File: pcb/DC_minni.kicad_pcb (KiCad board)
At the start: 4 copper layers, 72.2 x 87.7 mm, 60 parts, among them J1 DRUCKSENSOR, J2 Encoder, U1 ESP32-DevKitC, U2 USB-C to DIP PCB

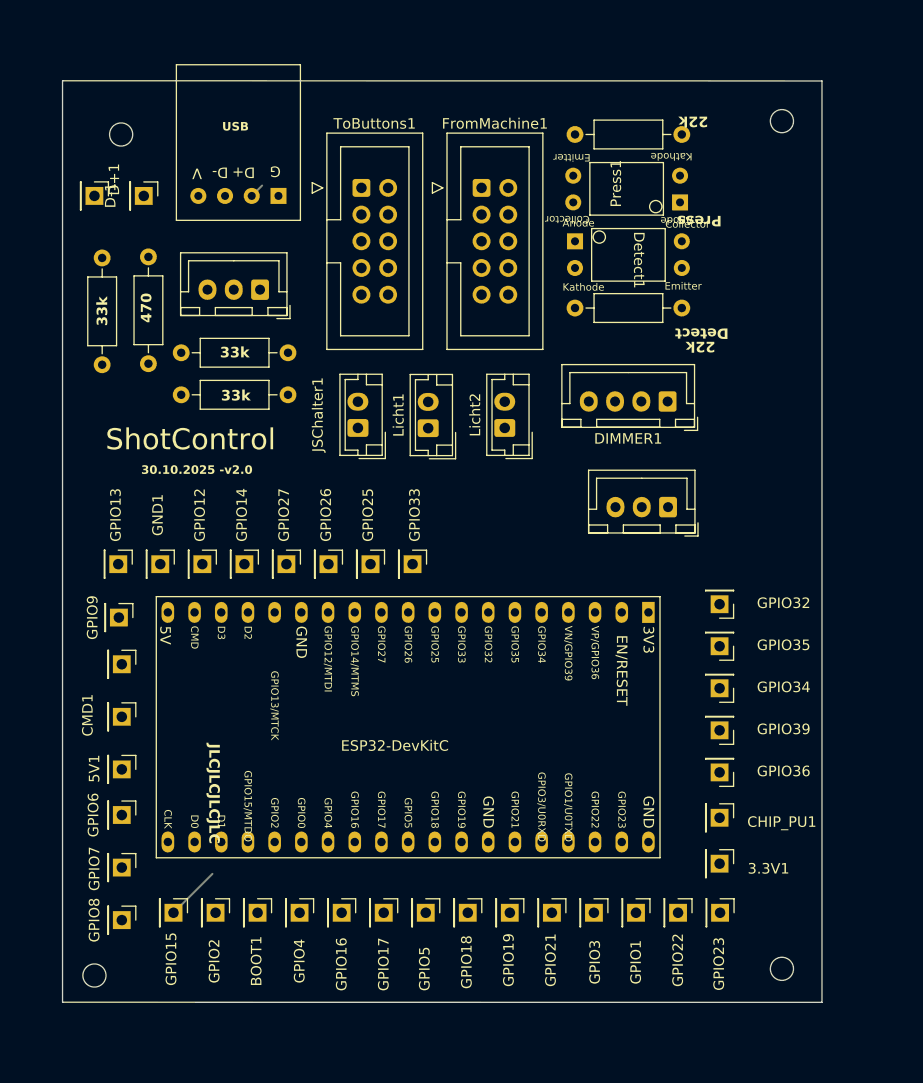
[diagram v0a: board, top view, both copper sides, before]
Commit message: PCB routing
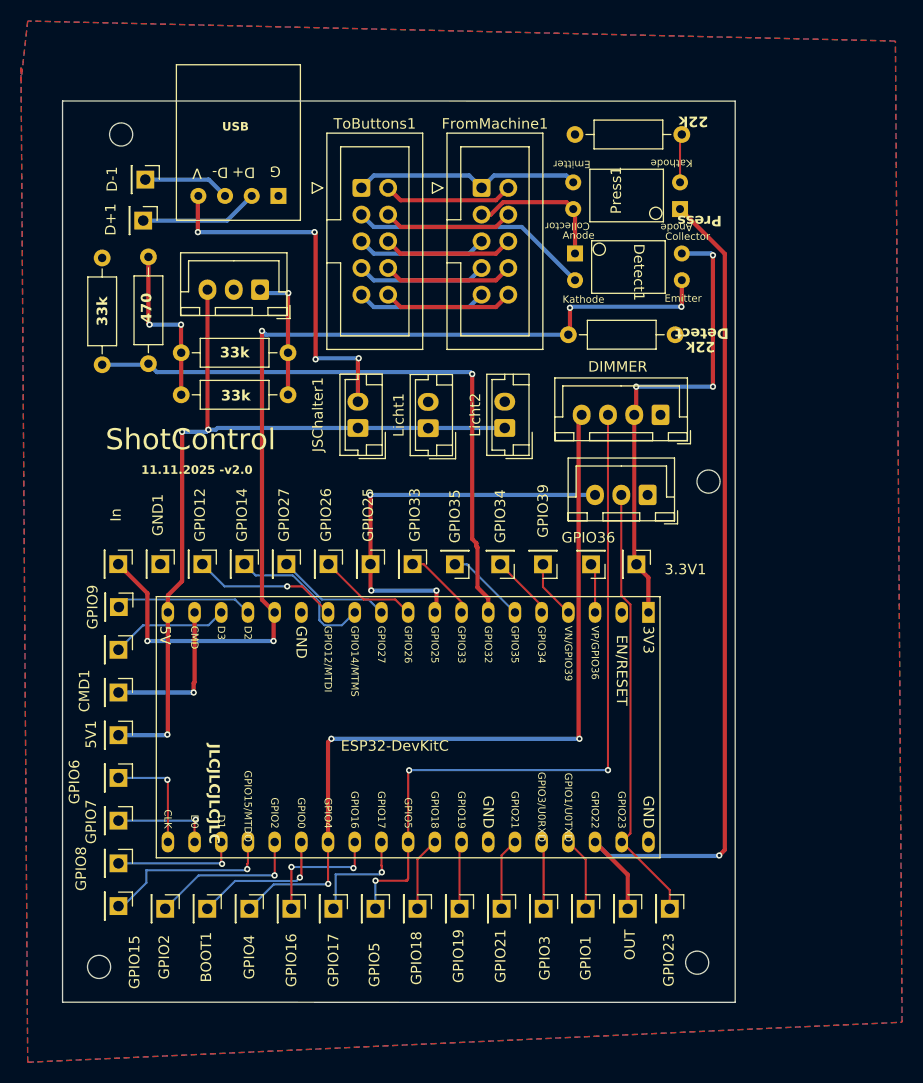
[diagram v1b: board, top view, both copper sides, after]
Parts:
- removed CHIP_PU1, GPIO32: Conn_01x01_Socket, Connector_PinHeader_2.54mm:PinHeader_1x01_P2.54mm_Vertical
- moved REF** 35.0 mm to (259.1, 113.0)
- moved 3.3V1 29.6 mm to (252.2, 120.9)
- moved GPIO35 26.4 mm to (234.9, 120.9)
- moved GPIO34 24.0 mm to (239.3, 120.9)
- moved GPIO36 23.3 mm to (247.9, 120.9)
- moved GPIO39 23.1 mm to (243.3, 120.9)
- moved REF** 8.09 mm to (258.0, 158.8)
- moved GPIO8 5.41 mm to (202.9, 149.4)
- moved GPIO15 5.27 mm to (202.9, 153.4)
- moved D+1 5.20 mm to (205.3, 88.2)
- moved BOOT1 4.80 mm to (211.4, 153.7)
- moved GPIO1 4.80 mm to (247.4, 153.7)
- moved GPIO16 4.80 mm to (219.4, 153.7)
- moved GPIO17 4.80 mm to (223.4, 153.7)
- moved GPIO18 4.80 mm to (231.4, 153.7)
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- renumbered DIMMER1 to DIMMER, GPIO13 to In, GPIO22 to OUT
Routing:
- net IN: track 0.00 -> 95.6 mm, vias 0 -> 5
- net OUT: track 0.00 -> 83.5 mm, vias 0 -> 1
- net +5V: track 0.00 -> 78.3 mm, vias 0 -> 3
- net ZeroCross: track 0.00 -> 77.0 mm, vias 0 -> 3
- net PWM: track 0.00 -> 69.2 mm, vias 0 -> 3
- net Drucksensor: track 0.40 -> 59.4 mm, vias 0 -> 1
- net +3.3V: track 0.71 -> 44.9 mm, vias 0 -> 3
- net Net-(GPIO23-Pin_1): track 0.00 -> 42.0 mm
- net Net-(GPIO25-Pin_1): track 0.00 -> 38.9 mm, vias 0 -> 3
- net Net-(JSChalter1-Pin_2): track 0.00 -> 35.0 mm, vias 0 -> 4
- net Net-(Detect1-Cathode): track 0.00 -> 22.9 mm
- net Net-(FromMachine1-Pin_1): track 0.00 -> 21.9 mm
- net Net-(RSP_01_1-Pad2): track 0.00 -> 16.2 mm, vias 0 -> 2
- net Net-(GPIO2-Pin_1): track 0.00 -> 14.9 mm, vias 0 -> 1
- net Net-(CMD1-Pin_1): track 0.00 -> 14.8 mm, vias 0 -> 1
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- added copper zone on B.Cu, net GND
- added copper zone on F.Cu, net GND
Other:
- board size 72.2 x 87.7 mm -> 64 x 85.8 mm
- board text added: "11.11.2025 -v2.0"
- board text removed: "30.10.2025 -v2.0"
- board text removed: "GPIO13/MTCK"
